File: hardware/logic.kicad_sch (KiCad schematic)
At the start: 15 parts, among them IC1 UCC2946DG4, U10 74LVC1G08, U8 74LVC1G08, U9 74LVC1G08

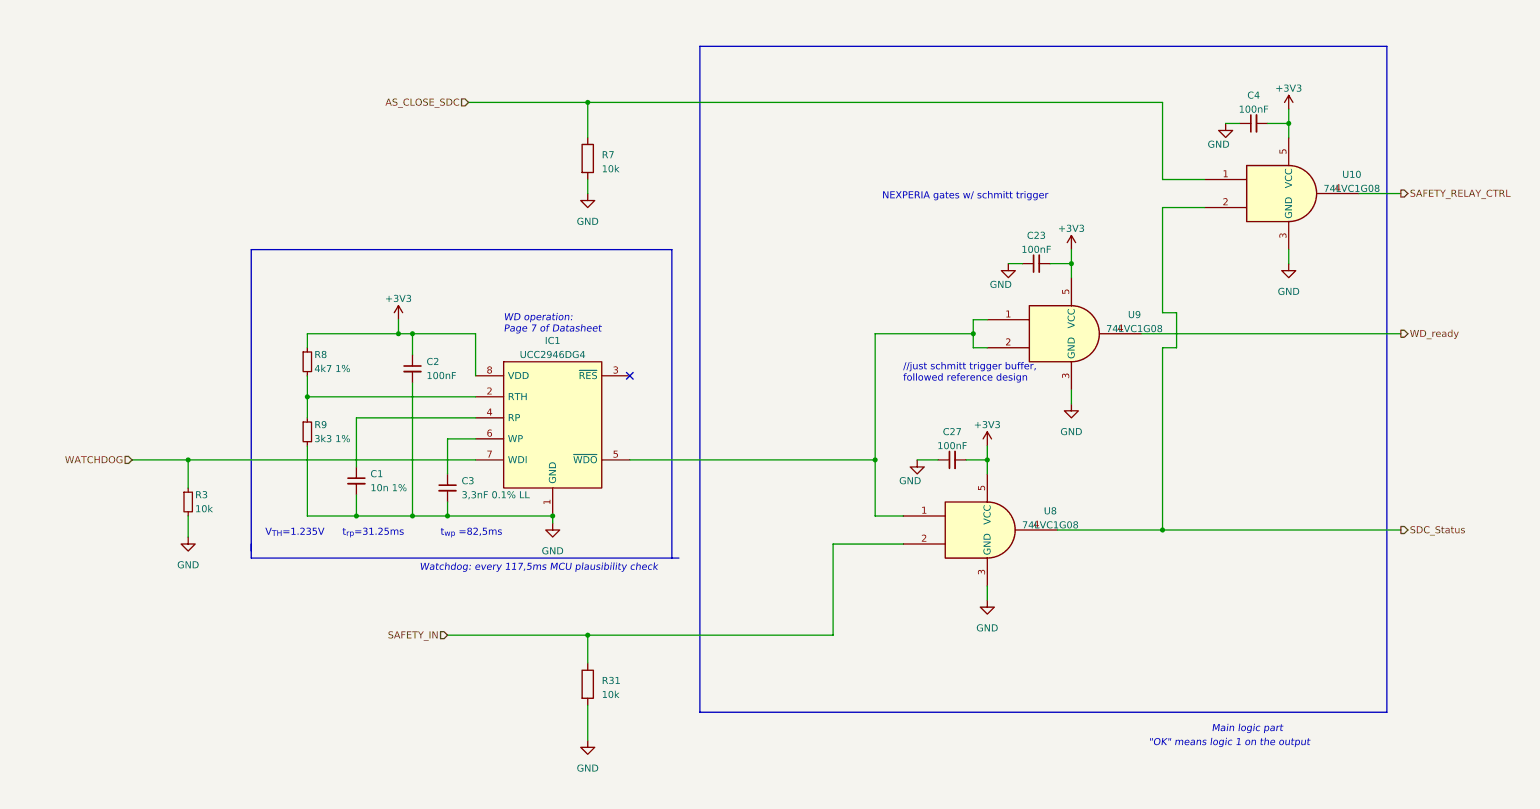
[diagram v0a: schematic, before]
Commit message: changed pcb version
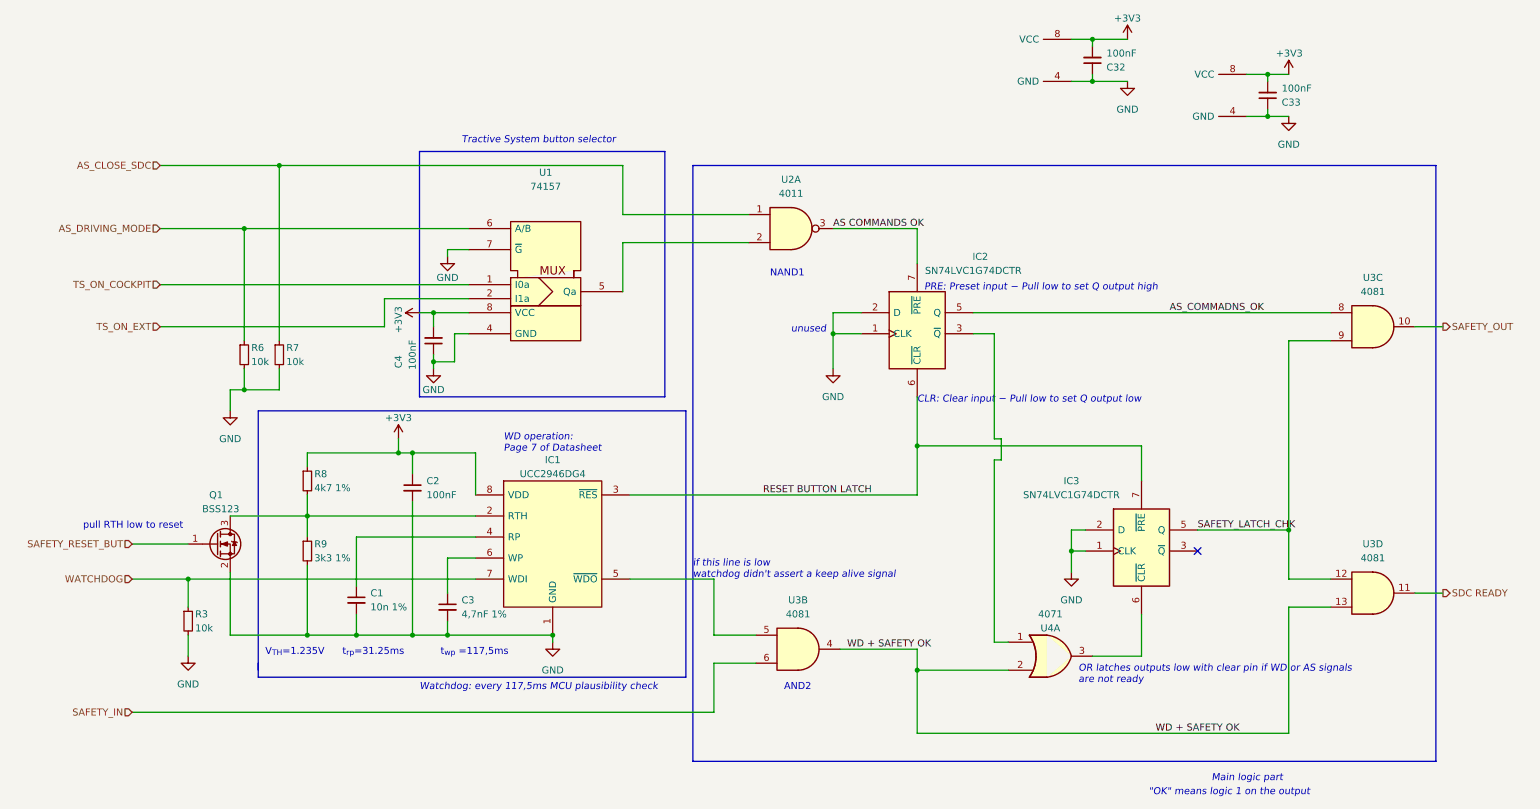
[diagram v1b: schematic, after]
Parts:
- removed C23, C27: 100nF, Capacitor_SMD:C_0603_1608Metric_Pad1.08x0.95mm_HandSolder, symbol Device:C_Small
- removed R31, R7: 10k, Resistor_SMD:R_0603_1608Metric_Pad0.98x0.95mm_HandSolder, symbol Device:R
- removed U10, U8, U9: 74LVC1G08, Package_TO_SOT_SMD:SOT-353_SC-70-5_Handsoldering, symbol 74xGxx:74LVC1G08
- added C32, C33: 100nF, Capacitor_SMD:C_0603_1608Metric_Pad1.08x0.95mm_HandSolder, symbol Device:C_Small
- added IC2, IC3: SN74LVC1G74DCTR, SamacSys_Parts:SOP65P400X130-8N, symbol SamacSys_Parts:SN74LVC1G74DCTR
- added Q1: BSS123, Package_TO_SOT_SMD:SOT-23, symbol Transistor_FET:BSS123
- added R6, R7: 10k, Resistor_SMD:R_0603_1608Metric_Pad0.98x0.95mm_HandSolder, symbol Device:R_Small
- added U1: 74157, Package_SO:VSSOP-8_2.3x2mm_P0.5mm, symbol 74xx_IEEE:74157
- added U2: 4011, Package_SO:TSSOP-14_4.4x5mm_P0.65mm, symbol 4xxx:4011
- added U3: 4081, Package_SO:TSSOP-14_4.4x5mm_P0.65mm, symbol 4xxx:4081
- added U4: 4071, Package_SO:TSSOP-14_4.4x5mm_P0.65mm, symbol 4xxx:4071
- C3: value 3,3nF 0.1% LL -> 4,7nF 1%
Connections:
- net +3V3: now also C32.2, C33.2, IC2.8 (VCC), IC3.8 (VCC), U1.8 (VCC)
- net AS_CLOSE_SDC: now also R7.1, U2.1
- net GND: now also C32.1, C33.1, IC2.1 (CLK), IC2.2 (D), IC2.4 (GND), IC3.1 (CLK), IC3.2 (D), IC3.4 (GND), Q1.2 (S), R6.2, R7.2, U1.4 (GND), U1.7 (~{G})
- net SAFETY_IN: now also U3.6
- net at IC1.2 (RTH), R8.2, R9.1: now also Q1.3 (D)
- net RESET BUTTON LATCH: now reaches IC1.3 (~{RES})
- net RESET BUTTON LATCH: now also IC2.6 (~{CLR}), IC3.7 (~{PRE})
- net at IC1.5 (~{WDO}): now also U3.5
- new net: IC2.3 (~{Q}), U4.1
- new net: IC3.6 (~{CLR}), U4.3
- new net: U1.5 (Qa), U2.2
- new net AS COMMANDS OK: IC2.7 (~{PRE}), U2.3
- new net AS_COMMADNS_OK: IC2.5 (Q), U3.8
- new net AS_DRIVING_MODE: R6.1, U1.6 (A/B)
- new net SAFETY_LATCH_CHK: IC3.5 (Q), U3.12, U3.9
- new net SAFETY_OUT: U3.10
- new net SAFETY_RESET_BUT: Q1.1 (G)
- new net SDC READY: U3.11
- new net TS_ON_COCKPIT: U1.1 (I0a)
- new net TS_ON_EXT: U1.2 (I1a)
- new net WD + SAFETY OK: U3.13, U3.4, U4.2
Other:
- note added: "AND2"
- note added: "CLR: Clear input − Pull low to set Q output low"
- note added: "NAND1"
- note added: "OR latches outputs low with clear pin if WD or AS signals are not ready"
- note added: "PRE: Preset input − Pull low to set Q output high"
- note added: "Tractive System button selector"
- note added: "if this line is low watchdog didn't assert a keep alive signal"
- note added: "pull RTH low to reset"
- note added: "t_{wp} =117,5ms"
- note added: "unused"
- note removed: "//just schmitt trigger buffer, followed reference design"
- note removed: "NEXPERIA gates w/ schmitt trigger"
- note removed: "t_{wp} =82,5ms"
- moved on the sheet: C1, C2, C3, IC1, R3, R8, R9

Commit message: uploaded older pcb version
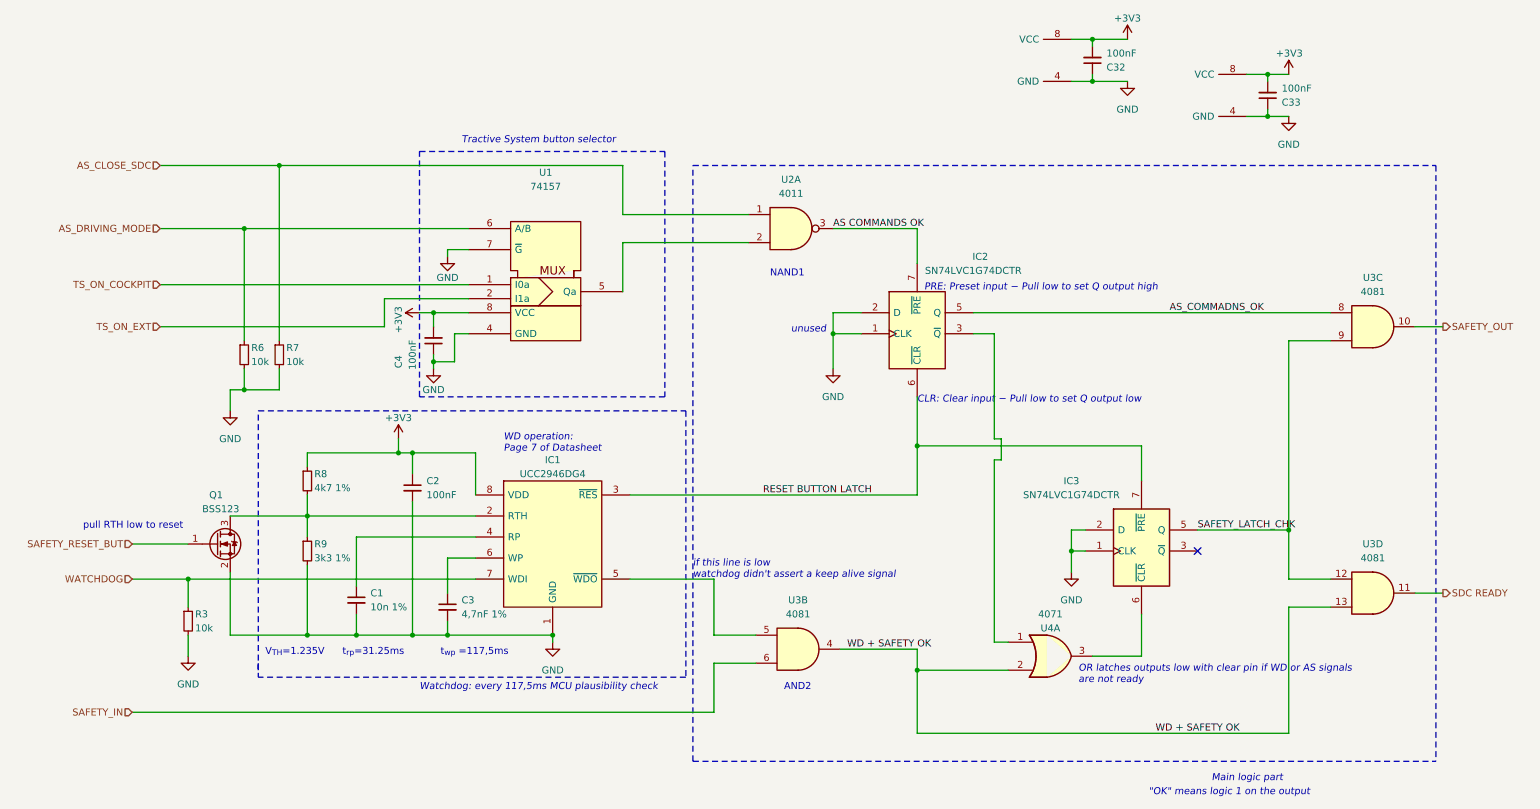
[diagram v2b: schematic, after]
